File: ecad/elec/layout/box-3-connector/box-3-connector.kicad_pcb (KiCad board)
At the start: 2 copper layers, 72.5 x 7.9 mm, 2 parts

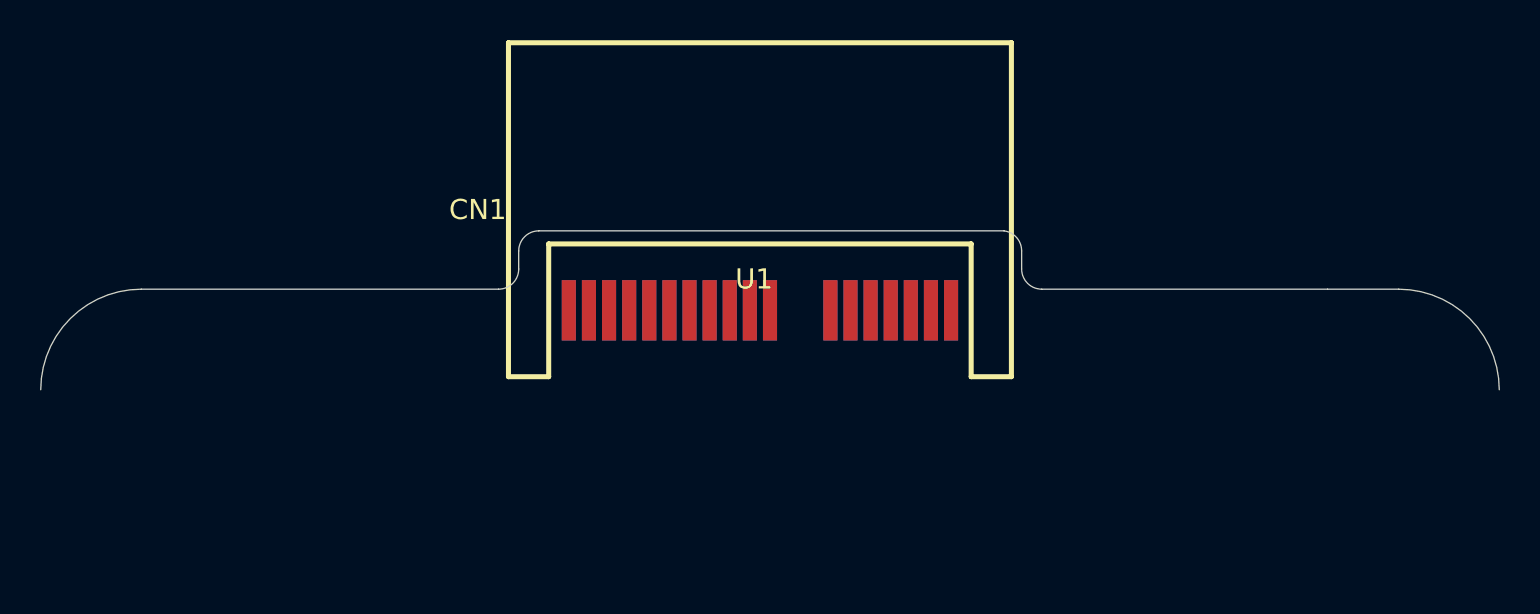
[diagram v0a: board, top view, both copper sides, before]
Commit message: improve workflow
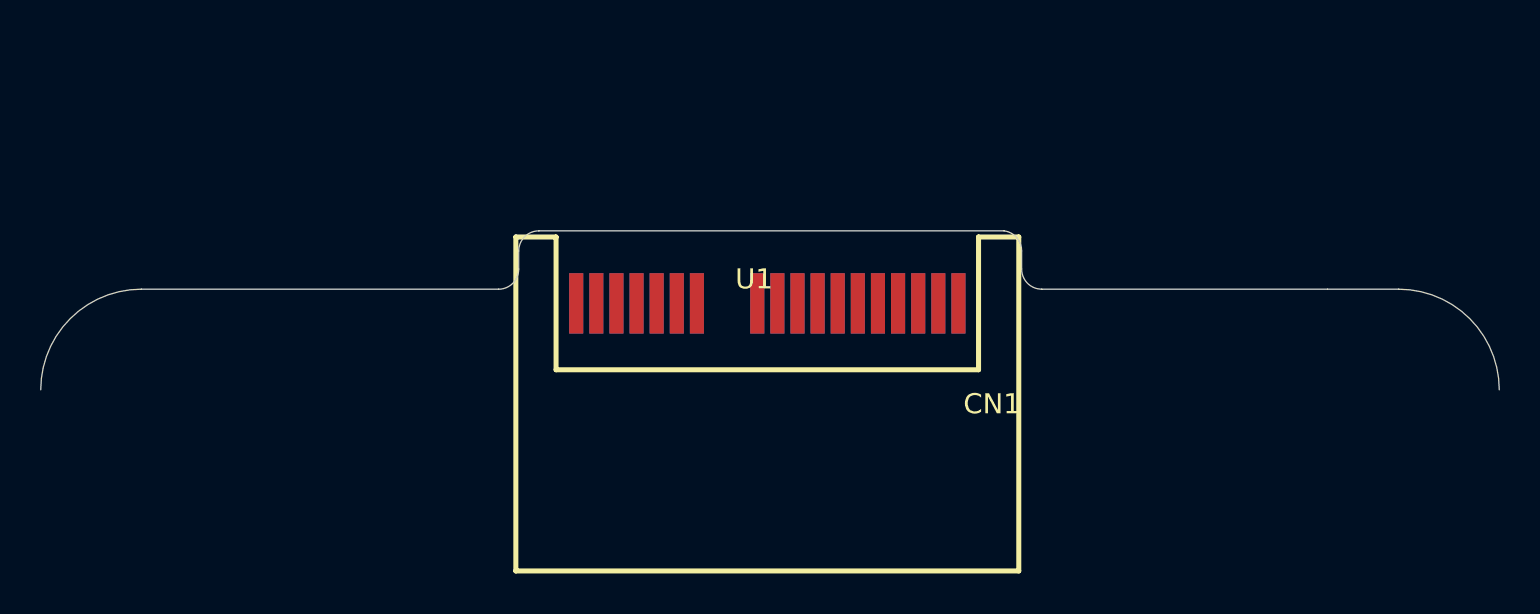
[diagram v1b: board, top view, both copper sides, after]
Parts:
- moved CN1 0.50 mm to (0.66, 0.71), turned to 180 degrees
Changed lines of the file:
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@@
 	(footprint "TE_Connectivity_5_1734857_1:CONN-SMD_5-1734857-1"
 		(layer "F.Cu")
-		(at 0.2921 1.05007)
+		(at 0.6585 0.7056 180)
 		(property "Reference" "CN1"
-			(at -12.6 -5 0)
+			(at -12.6 -5 180)
 			(layer "F.SilkS")
 			(effects
@@
 		)
 		(property "Value" ""
-			(at 0 4 0)
+			(at 0 4 180)
 			(layer "F.Fab")
 			(effects
@@
 		)
 		(property "Datasheet" ""
-			(at 0 0 0)
+			(at 0 0 180)
 			(layer "F.Fab")
 			(hide yes)
@@
 		)
 		(property "Description" ""
-			(at 0 0 0)
+			(at 0 0 180)
 			(layer "F.Fab")
 			(hide yes)
@@
 		)
 		(property "LCSC" "C4645333"
-			(at 0 0 0)
+			(at 0 0 180)
 			(layer "User.9")
 			(hide yes)
@@
 		)
 		(property "Manufacturer" "TE Connectivity"
-			(at 0 0 0)
+			(at 0 0 180)
 			(layer "User.9")
 			(hide yes)
@@
 		)
 		(property "Partnumber" "5-1734857-1"
-			(at 0 0 0)
+			(at 0 0 180)
 			(layer "User.9")
 			(hide yes)
@@
 		)
 		(property "atopile_address" "conn"
-			(at 0 0 0)
+			(at 0 0 180)
 			(layer "User.9")
 			(hide yes)
@@
 		)
 		(property "lcsc_id" "C4645333"
-			(at 0 0 0)
+			(at 0 0 180)
 			(layer "User.9")
 			(hide yes)
@@
 		)
 		(pad "A1" smd rect
-			(at -9.5 0 0)
+			(at -9.5 0 180)
 			(size 0.7 3)
 			(layers "F.Cu" "F.Paste" "F.Mask")
@@
 		)
 		(pad "A2" smd rect
-			(at -8.5 0 0)
+			(at -8.5 0 180)
 			(size 0.7 3)
 			(layers "F.Cu" "F.Paste" "F.Mask")
@@
 		)
 		(pad "A3" smd rect
-			(at -7.5 0 0)
+			(at -7.5 0 180)
 			(size 0.7 3)
 			(layers "F.Cu" "F.Paste" "F.Mask")
@@
 		)
 		(pad "A4" smd rect
-			(at -6.5 0 0)
+			(at -6.5 0 180)
 			(size 0.7 3)
 			(layers "F.Cu" "F.Paste" "F.Mask")
@@
 		)
 		(pad "A5" smd rect
-			(at -5.5 0 0)
+			(at -5.5 0 180)
 			(size 0.7 3)
 			(layers "F.Cu" "F.Paste" "F.Mask")
@@
 		)
 		(pad "A6" smd rect
-			(at -4.5 0 0)
+			(at -4.5 0 180)
 			(size 0.7 3)
 			(layers "F.Cu" "F.Paste" "F.Mask")
@@
 		)
 		(pad "A7" smd rect
-			(at -3.5 0 0)
+			(at -3.5 0 180)
 			(size 0.7 3)
 			(layers "F.Cu" "F.Paste" "F.Mask")
@@
 		)
 		(pad "A8" smd rect
-			(at -2.5 0 0)
+			(at -2.5 0 180)
 			(size 0.7 3)
 			(layers "F.Cu" "F.Paste" "F.Mask")
@@
 		)
 		(pad "A9" smd rect
-			(at -1.5 0 0)
+			(at -1.5 0 180)
 			(size 0.7 3)
 			(layers "F.Cu" "F.Paste" "F.Mask")
@@
 		)
 		(pad "A10" smd rect
-			(at -0.5 0 0)
+			(at -0.5 0 180)
 			(size 0.7 3)
 			(layers "F.Cu" "F.Paste" "F.Mask")
@@
 		)
 		(pad "A11" smd rect
-			(at 0.5 0 0)
+			(at 0.5 0 180)
 			(size 0.7 3)
 			(layers "F.Cu" "F.Paste" "F.Mask")
@@
 		)
 		(pad "A12" smd rect
-			(at 3.5 0 0)
+			(at 3.5 0 180)
 			(size 0.7 3)
 			(layers "F.Cu" "F.Paste" "F.Mask")
@@
 		)
 		(pad "A13" smd rect
-			(at 4.5 0 0)
+			(at 4.5 0 180)
 			(size 0.7 3)
 			(layers "F.Cu" "F.Paste" "F.Mask")
@@
 		)
 		(pad "A14" smd rect
-			(at 5.5 0 0)
+			(at 5.5 0 180)
 			(size 0.7 3)
 			(layers "F.Cu" "F.Paste" "F.Mask")
@@
 		)
 		(pad "A15" smd rect
-			(at 6.5 0 0)
+			(at 6.5 0 180)
 			(size 0.7 3)
 			(layers "F.Cu" "F.Paste" "F.Mask")
@@
 		)
 		(pad "A16" smd rect
-			(at 7.5 0 0)
+			(at 7.5 0 180)
 			(size 0.7 3)
 			(layers "F.Cu" "F.Paste" "F.Mask")
@@
 		)
 		(pad "A17" smd rect
-			(at 8.5 0 0)
+			(at 8.5 0 180)
 			(size 0.7 3)
 			(layers "F.Cu" "F.Paste" "F.Mask")
@@
 		)
 		(pad "A18" smd rect
-			(at 9.5 0 0)
+			(at 9.5 0 180)
 			(size 0.7 3)
 			(layers "F.Cu" "F.Paste" "F.Mask")
@@
 		)
 		(pad "B1" smd rect
-			(at -9.5 0 0)
+			(at -9.5 0 180)
 			(size 0.7 3)
 			(layers "B.Cu" "B.Paste" "B.Mask")
@@
 		)
 		(pad "B2" smd rect
-			(at -8.5 0 0)
+			(at -8.5 0 180)
 			(size 0.7 3)
 			(layers "B.Cu" "B.Paste" "B.Mask")
@@
 		)
 		(pad "B3" smd rect
-			(at -7.5 0 0)
+			(at -7.5 0 180)
 			(size 0.7 3)
 			(layers "B.Cu" "B.Paste" "B.Mask")
@@
 		)
 		(pad "B4" smd rect
-			(at -6.5 0 0)
+			(at -6.5 0 180)
 			(size 0.7 3)
 			(layers "B.Cu" "B.Paste" "B.Mask")
@@
 		)
 		(pad "B5" smd rect
-			(at -5.5 0 0)
+			(at -5.5 0 180)
 			(size 0.7 3)
 			(layers "B.Cu" "B.Paste" "B.Mask")
@@
 		)
 		(pad "B6" smd rect
-			(at -4.5 0 0)
+			(at -4.5 0 180)
 			(size 0.7 3)
 			(layers "B.Cu" "B.Paste" "B.Mask")
@@
 		)
 		(pad "B7" smd rect
-			(at -3.5 0 0)
+			(at -3.5 0 180)
 			(size 0.7 3)
 			(layers "B.Cu" "B.Paste" "B.Mask")
@@
 		)
 		(pad "B8" smd rect
-			(at -2.5 0 0)
+			(at -2.5 0 180)
 			(size 0.7 3)
 			(layers "B.Cu" "B.Paste" "B.Mask")
@@
 		)
 		(pad "B9" smd rect
-			(at -1.5 0 0)
+			(at -1.5 0 180)
 			(size 0.7 3)
 			(layers "B.Cu" "B.Paste" "B.Mask")
@@
 		)
 		(pad "B10" smd rect
-			(at -0.5 0 0)
+			(at -0.5 0 180)
 			(size 0.7 3)
 			(layers "B.Cu" "B.Paste" "B.Mask")
@@
 		)
 		(pad "B11" smd rect
-			(at 0.5 0 0)
+			(at 0.5 0 180)
 			(size 0.7 3)
 			(layers "B.Cu" "B.Paste" "B.Mask")
@@
 		)
 		(pad "B12" smd rect
-			(at 3.5 0 0)
+			(at 3.5 0 180)
 			(size 0.7 3)
 			(layers "B.Cu" "B.Paste" "B.Mask")
@@
 		)
 		(pad "B13" smd rect
-			(at 4.5 0 0)
+			(at 4.5 0 180)
 			(size 0.7 3)
 			(layers "B.Cu" "B.Paste" "B.Mask")
@@
 		)
 		(pad "B14" smd rect
-			(at 5.5 0 0)
+			(at 5.5 0 180)
 			(size 0.7 3)
 			(layers "B.Cu" "B.Paste" "B.Mask")
@@
 		)
 		(pad "B15" smd rect
-			(at 6.5 0 0)
+			(at 6.5 0 180)
 			(size 0.7 3)
 			(layers "B.Cu" "B.Paste" "B.Mask")
@@
 		)
 		(pad "B16" smd rect
-			(at 7.5 0 0)
+			(at 7.5 0 180)
 			(size 0.7 3)
 			(layers "B.Cu" "B.Paste" "B.Mask")
@@
 		)
 		(pad "B17" smd rect
-			(at 8.5 0 0)
+			(at 8.5 0 180)
 			(size 0.7 3)
 			(layers "B.Cu" "B.Paste" "B.Mask")
@@
 		)
 		(pad "B18" smd rect
-			(at 9.5 0 0)
-			(size 0.7 3)
-			(layers "B.Cu" "B.Paste" "B.Mask")
+			(at 9.5 0 180)
+			(size 0.7 3)
+			(layers "B.Cu" "B.Paste" "B.Mask")
